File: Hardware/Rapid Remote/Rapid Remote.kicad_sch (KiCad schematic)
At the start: 42 parts, among them J1 Conn_01x02_Socket, U1 MIC5504-3.3YM5, U2 ESP32-C3-MINI-1-N4, U3 WS4518D, U4 XB6096I2SV

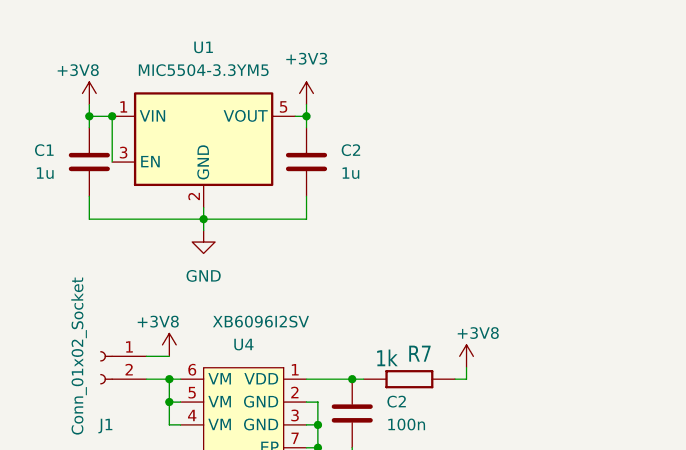
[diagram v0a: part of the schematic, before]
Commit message: updated gpio values
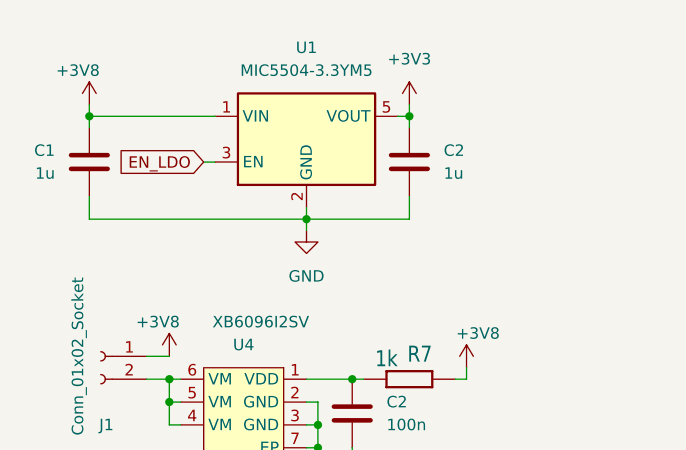
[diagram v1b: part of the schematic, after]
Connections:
- net +3V8: no longer U1.3 (EN)
- net EN_LDO: now also U1.3 (EN)
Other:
- moved on the sheet: C2, U1
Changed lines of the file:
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@@
   (junction (at 251.46 88.9) (diameter 0) (color 0 0 0 0)
   )
-  (junction (at 34.29 34.29) (diameter 0) (color 0 0 0 0)
+  (junction (at 45.72 34.29) (diameter 0) (color 0 0 0 0)
   )
   (junction (at 35.56 181.61) (diameter 0) (color 0 0 0 0)
   )
-  (junction (at 24.13 22.86) (diameter 0) (color 0 0 0 0)
-  )
   (junction (at 251.46 99.06) (diameter 0) (color 0 0 0 0)
   )
@@
   (junction (at 95.25 29.21) (diameter 0) (color 0 0 0 0)
   )
-  (junction (at 45.72 22.86) (diameter 0) (color 0 0 0 0)
+  (junction (at 57.15 22.86) (diameter 0) (color 0 0 0 0)
   )
   (junction (at 30.48 154.94) (diameter 0) (color 0 0 0 0)
@@
     (stroke (width 0.1524) (type solid))
   )
+  (wire (pts (xy 21.59 34.29) (xy 45.72 34.29))
+    (stroke (width 0) (type default))
+  )
   (wire (pts (xy 187.96 78.74) (xy 189.23 78.74))
     (stroke (width 0) (type default))
@@
     (stroke (width 0.1524) (type solid))
   )
-  (wire (pts (xy 45.72 34.29) (xy 34.29 34.29))
+  (wire (pts (xy 57.15 34.29) (xy 45.72 34.29))
     (stroke (width 0) (type default))
   )
@@
     (stroke (width 0) (type default))
   )
-  (wire (pts (xy 24.13 22.86) (xy 21.59 22.86))
-    (stroke (width 0) (type default))
-  )
   (wire (pts (xy 30.48 57.15) (xy 30.48 54.61))
     (stroke (width 0) (type default))
@@
     (stroke (width 0.1524) (type solid))
   )
-  (wire (pts (xy 45.72 22.86) (xy 45.72 24.13))
+  (wire (pts (xy 57.15 22.86) (xy 57.15 24.13))
     (stroke (width 0) (type default))
   )
@@
     (stroke (width 0.1524) (type solid))
   )
-  (wire (pts (xy 44.45 22.86) (xy 45.72 22.86))
+  (wire (pts (xy 55.88 22.86) (xy 57.15 22.86))
     (stroke (width 0) (type default))
   )
@@
     (stroke (width 0) (type default))
   )
+  (wire (pts (xy 21.59 34.29) (xy 21.59 31.75))
+    (stroke (width 0) (type default))
+  )
   (wire (pts (xy 123.19 80.01) (xy 124.46 80.01))
     (stroke (width 0) (type default))
@@
     (stroke (width 0.1524) (type solid))
   )
-  (wire (pts (xy 21.59 31.75) (xy 21.59 34.29))
+  (wire (pts (xy 34.29 27.94) (xy 35.56 27.94))
     (stroke (width 0) (type default))
   )
@@
     (stroke (width 0) (type default))
   )
-  (wire (pts (xy 21.59 34.29) (xy 34.29 34.29))
-    (stroke (width 0) (type default))
-  )
   (wire (pts (xy 29.21 189.23) (xy 35.56 189.23))
     (stroke (width 0) (type default))
@@
     (stroke (width 0.1524) (type solid))
   )
-  (wire (pts (xy 24.13 27.94) (xy 24.13 22.86))
-    (stroke (width 0) (type default))
-  )
-  (wire (pts (xy 45.72 31.75) (xy 45.72 34.29))
+  (wire (pts (xy 57.15 31.75) (xy 57.15 34.29))
     (stroke (width 0) (type default))
   )
@@
     (stroke (width 0) (type default))
   )
-  (wire (pts (xy 34.29 33.02) (xy 34.29 34.29))
+  (wire (pts (xy 45.72 33.02) (xy 45.72 34.29))
     (stroke (width 0) (type default))
   )
@@
     (stroke (width 0) (type default))
   )
-  (wire (pts (xy 34.29 35.56) (xy 34.29 34.29))
+  (wire (pts (xy 45.72 35.56) (xy 45.72 34.29))
     (stroke (width 0) (type default))
   )
@@
     (stroke (width 0) (type default))
   )
-  (wire (pts (xy 45.72 22.86) (xy 45.72 21.59))
+  (wire (pts (xy 57.15 22.86) (xy 57.15 21.59))
     (stroke (width 0) (type default))
   )
   (wire (pts (xy 250.19 68.58) (xy 251.46 68.58))
+    (stroke (width 0) (type default))
+  )
+  (wire (pts (xy 21.59 22.86) (xy 35.56 22.86))
     (stroke (width 0) (type default))
   )
@@
     (effects (font (size 1.27 1.27)) (justify right))
     (property "Intersheetrefs" "${INTERSHEET_REFS}" (at 178.0994 55.88 0)
+      (effects (font (size 1.27 1.27)) (justify right) hide)
+    )
+  )
+  (global_label "EN_LDO" (shape input) (at 34.29 27.94 180) (fields_autoplaced)
+    (effects (font (size 1.27 1.27)) (justify right))
+    (property "Intersheetrefs" "${INTERSHEET_REFS}" (at 24.2291 27.94 0)
       (effects (font (size 1.27 1.27)) (justify right) hide)
     )
@@
     )
   )
-  (symbol (lib_id "Regulator_Linear:MIC5504-3.3YM5") (at 34.29 25.4 0) (unit 1)
+  (symbol (lib_id "Regulator_Linear:MIC5504-3.3YM5") (at 45.72 25.4 0) (unit 1)
     (in_bom yes) (on_board yes) (dnp no) (fields_autoplaced)
-    (property "Reference" "U1" (at 34.29 15.24 0)
-      (effects (font (size 1.27 1.27)))
-    )
-    (property "Value" "MIC5504-3.3YM5" (at 34.29 17.78 0)
-      (effects (font (size 1.27 1.27)))
-    )
-    (property "Footprint" "Package_TO_SOT_SMD:SOT-23-5" (at 34.29 35.56 0)
-      (effects (font (size 1.27 1.27)) hide)
-    )
-    (property "Datasheet" "http://ww1.microchip.com/downloads/en/DeviceDoc/MIC550X.pdf" (at 27.94 19.05 0)
+    (property "Reference" "U1" (at 45.72 15.24 0)
+      (effects (font (size 1.27 1.27)))
+    )
+    (property "Value" "MIC5504-3.3YM5" (at 45.72 17.78 0)
+      (effects (font (size 1.27 1.27)))
+    )
+    (property "Footprint" "Package_TO_SOT_SMD:SOT-23-5" (at 45.72 35.56 0)
+      (effects (font (size 1.27 1.27)) hide)
+    )
+    (property "Datasheet" "http://ww1.microchip.com/downloads/en/DeviceDoc/MIC550X.pdf" (at 39.37 19.05 0)
       (effects (font (size 1.27 1.27)) hide)
     )
@@
     )
   )
-  (symbol (lib_name "GND_3") (lib_id "power:GND") (at 34.29 35.56 0) (unit 1)
+  (symbol (lib_name "GND_3") (lib_id "power:GND") (at 45.72 35.56 0) (unit 1)
     (in_bom yes) (on_board yes) (dnp no) (fields_autoplaced)
-    (property "Reference" "#PWR010" (at 34.29 41.91 0)
-      (effects (font (size 1.27 1.27)) hide)
-    )
-    (property "Value" "GND" (at 34.29 40.64 0)
-      (effects (font (size 1.27 1.27)))
-    )
-    (property "Footprint" "" (at 34.29 35.56 0)
-      (effects (font (size 1.27 1.27)) hide)
-    )
-    (property "Datasheet" "" (at 34.29 35.56 0)
+    (property "Reference" "#PWR010" (at 45.72 41.91 0)
+      (effects (font (size 1.27 1.27)) hide)
+    )
+    (property "Value" "GND" (at 45.72 40.64 0)
+      (effects (font (size 1.27 1.27)))
+    )
+    (property "Footprint" "" (at 45.72 35.56 0)
+      (effects (font (size 1.27 1.27)) hide)
+    )
+    (property "Datasheet" "" (at 45.72 35.56 0)
       (effects (font (size 1.27 1.27)) hide)
     )
@@
     )
   )
-  (symbol (lib_id "Device:C") (at 45.72 27.94 0) (unit 1)
+  (symbol (lib_id "Device:C") (at 57.15 27.94 0) (unit 1)
     (in_bom yes) (on_board yes) (dnp no) (fields_autoplaced)
-    (property "Reference" "C2" (at 49.53 26.67 0)
+    (property "Reference" "C2" (at 60.96 26.67 0)
       (effects (font (size 1.27 1.27)) (justify left))
     )
-    (property "Value" "1u" (at 49.53 29.21 0)
+    (property "Value" "1u" (at 60.96 29.21 0)
       (effects (font (size 1.27 1.27)) (justify left))
     )
-    (property "Footprint" "Capacitor_SMD:C_0603_1608Metric" (at 46.6852 31.75 0)
-      (effects (font (size 1.27 1.27)) hide)
-    )
-    (property "Datasheet" "~" (at 45.72 27.94 0)
+    (property "Footprint" "Capacitor_SMD:C_0603_1608Metric" (at 58.1152 31.75 0)
+      (effects (font (size 1.27 1.27)) hide)
+    )
+    (property "Datasheet" "~" (at 57.15 27.94 0)
       (effects (font (size 1.27 1.27)) hide)
     )
@@
     )
   )
-  (symbol (lib_id "power:+3V3") (at 45.72 21.59 0) (unit 1)
+  (symbol (lib_id "power:+3V3") (at 57.15 21.59 0) (unit 1)
     (in_bom yes) (on_board yes) (dnp no) (fields_autoplaced)
-    (property "Reference" "#PWR01" (at 45.72 25.4 0)
-      (effects (font (size 1.27 1.27)) hide)
-    )
-    (property "Value" "+3V3" (at 45.72 16.51 0)
-      (effects (font (size 1.27 1.27)))
-    )
-    (property "Footprint" "" (at 45.72 21.59 0)
-      (effects (font (size 1.27 1.27)) hide)
-    )
-    (property "Datasheet" "" (at 45.72 21.59 0)
-      (effects (font (size 1.27 1.27)) hide)
-    )
+    (property "Reference" "#PWR01" (at 57.15 25.4 0)
+      (effects (font (size 1.27 1.27)) hide)
+    )
+    (property "Value" "+3V3" (at 57.15 16.51 0)
+      (effects (font (size 1.27 1.27)))
+    )
+    (property "Footprint" "" (at 57.15 21.59 0)
+      (effects (font (size 1.27 1.27)) hide)
+    )
+    (property "Datasheet" "" (at 57.15 21.59 0)
+      (effects (font (size 1.27 1.27)) hide)
+    )
